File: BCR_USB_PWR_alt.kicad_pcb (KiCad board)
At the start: 2 copper layers, 13.4 x 21.8 mm, 2 parts, among them CN1 DB9_Female, CN2 UE27AC54100

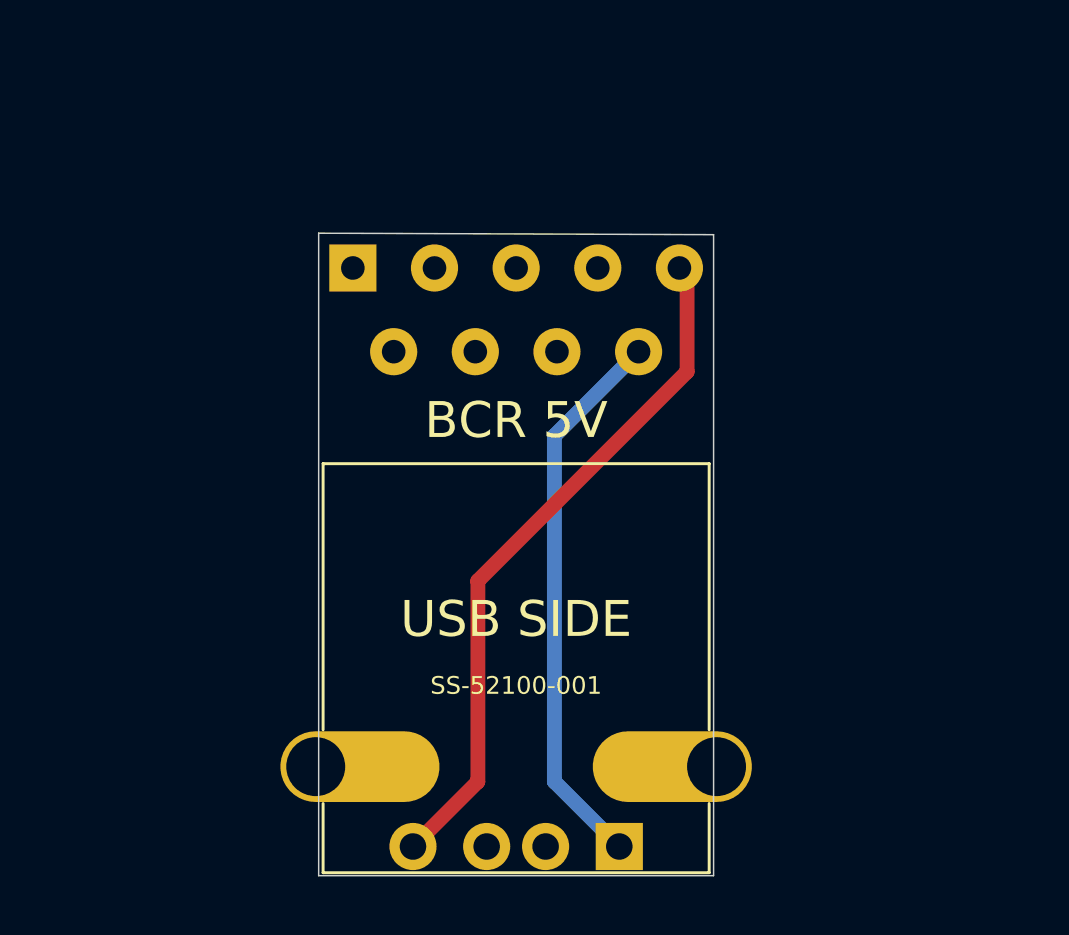
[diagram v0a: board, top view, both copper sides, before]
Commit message: clean up junk files
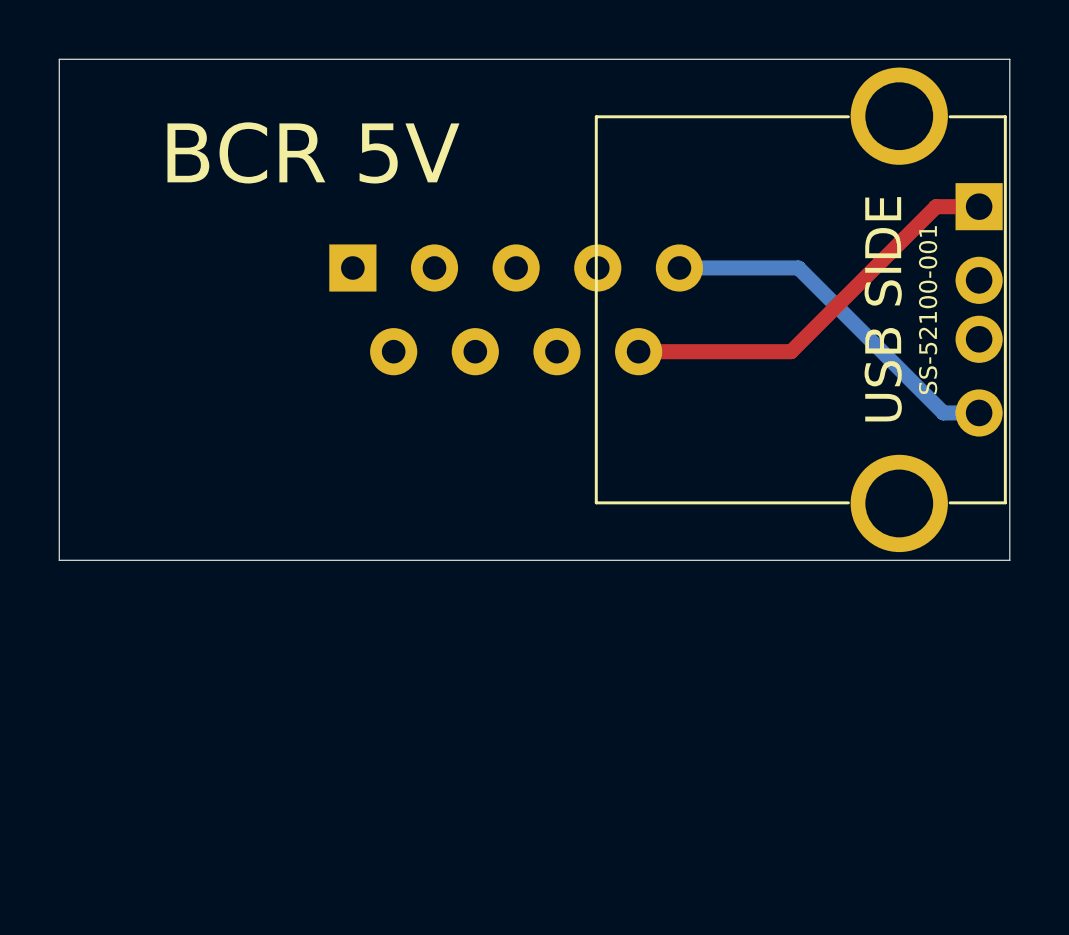
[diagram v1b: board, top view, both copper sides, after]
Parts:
- CN1: footprint 0_LOCAL:TE-5207826_nec -> 0_LOCAL:TE-5207826
- CN2: footprint 0_LOCAL:USB_A_Female_UE27AC54100_cut -> 0_LOCAL:USB_A_Female_UE27AC54100
- moved CN2 20.2 mm to (140.0, 95.8), turned to 270 degrees
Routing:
- net /GND: track 23.6 -> 12.2 mm
- net /+5V: track 18.9 -> 13.6 mm
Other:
- board size 13.4 x 21.8 mm -> 32.2 x 17 mm
- board text added: "5v USB power from BCR port"
- board text added: "TE 5207826"
- board text removed: "5v USB power"
- board text removed: "A-DF 09 PP/Z"
- board text removed: "NEC PC-8201 / PC-8300"
- board text removed: "from BCR port"
